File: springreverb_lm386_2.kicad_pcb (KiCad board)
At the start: 2 copper layers, 69.9 x 55.3 mm, 49 parts, among them J1 IN, J10 FromSW, J13 FromGND, J14 From, J15 VR_3_1, J16 VR4_1, J2 Vin, J3 GND, J4 VR1_3, J5 toC6, J6 toC7, J7 VR2_3, J8 VR_2_2, J9 To, U1 TL072, U2 TC1044S, U3 LM386

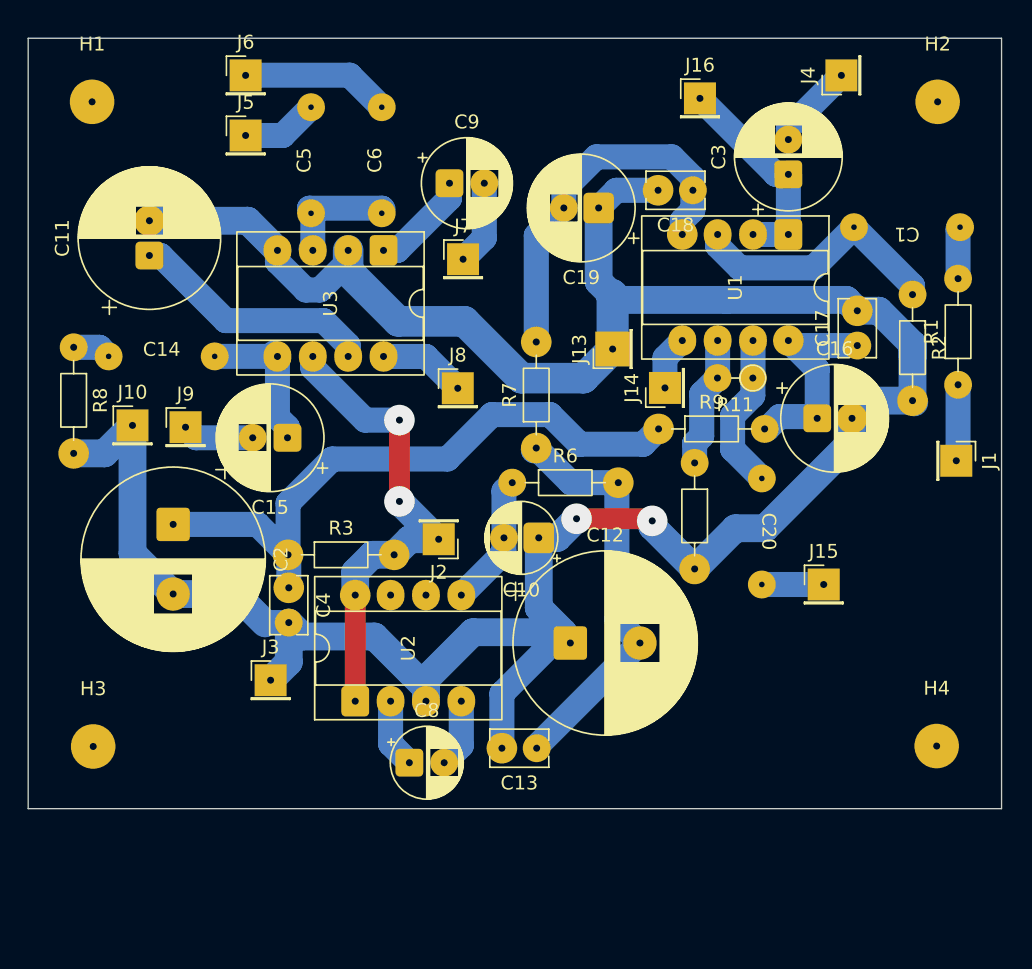
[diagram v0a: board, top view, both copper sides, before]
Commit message: 一旦配置完了
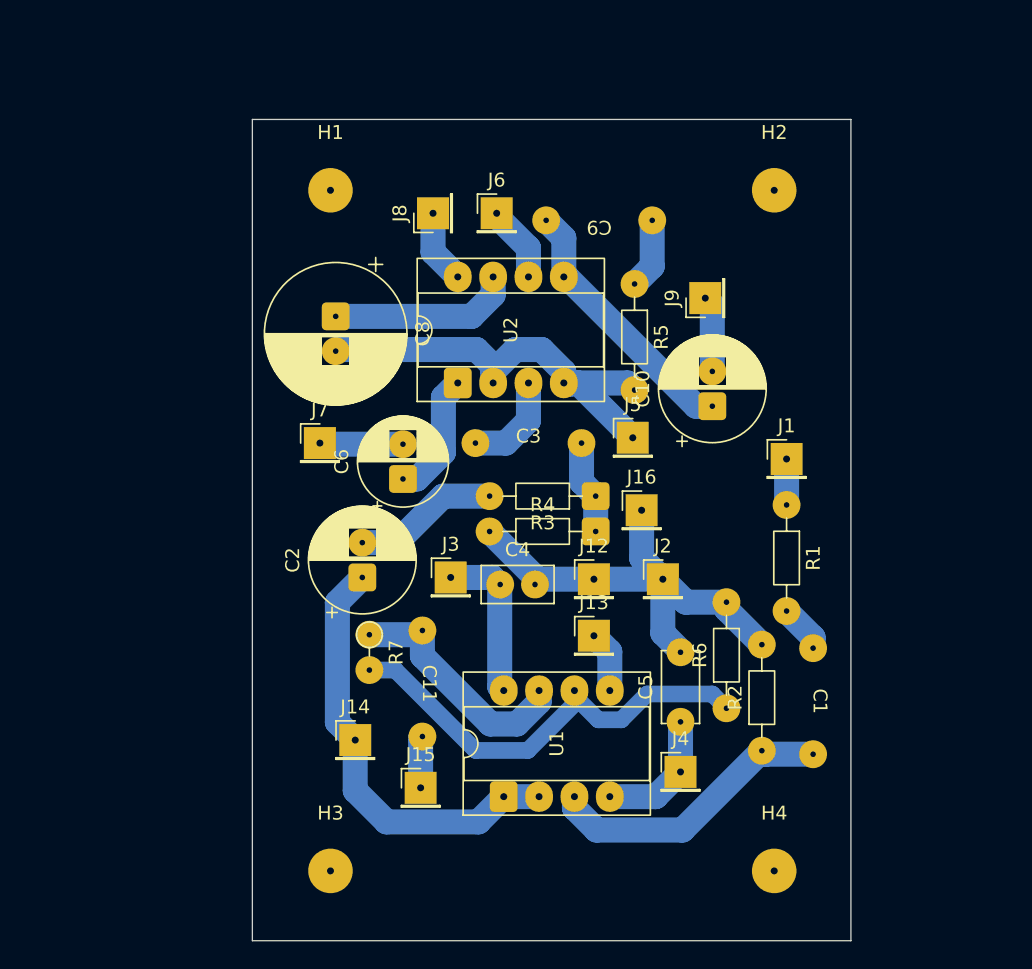
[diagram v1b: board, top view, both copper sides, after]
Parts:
- removed C12: 1000u, Capacitor_THT:CP_Radial_D13.0mm_P5.00mm
- removed C13, C17, C18: 0.1u, Capacitor_THT:C_Rect_L4.0mm_W2.5mm_P2.50mm
- removed C14: 0.047u, MyLibrary:9.3_4.3_p7.5
- removed C15, C16, C19: 100u, Capacitor_THT:CP_Radial_D7.5mm_P2.50mm
- removed C20: 0.022uF, MyLibrary:9.3_4.3_p7.5
- removed J10: FromSW, MyLibrary:PinHeader_1x01_P2.54mm_Vertical
- removed R10: 2.2k, Resistor_THT:R_Axial_DIN0204_L3.6mm_D1.6mm_P7.62mm_Horizontal
- removed R11: 220k, Resistor_THT:R_Axial_DIN0204_L3.6mm_D1.6mm_P2.54mm_Vertical
- removed R8: 10, Resistor_THT:R_Axial_DIN0204_L3.6mm_D1.6mm_P7.62mm_Horizontal
- removed R9: 470, Resistor_THT:R_Axial_DIN0204_L3.6mm_D1.6mm_P7.62mm_Horizontal
- removed U3: LM386, MyLibrary:CERDIP-8_W7.62mm_SideBrazed_Socket
- added J12: FromGND, MyLibrary:PinHeader_1x01_P2.54mm_Vertical, F.Cu at (89.5, 105.0)
- added R4: 4k, Resistor_THT:R_Axial_DIN0204_L3.6mm_D1.6mm_P7.62mm_Horizontal, F.Cu at (82.0, 101.6)
- added R5: 10, Resistor_THT:R_Axial_DIN0204_L3.6mm_D1.6mm_P7.62mm_Horizontal, F.Cu at (92.5, 83.8)
- C10: value 10u -> 100u; footprint Capacitor_THT:CP_Radial_D5.0mm_P2.50mm -> Capacitor_THT:CP_Radial_D7.5mm_P2.50mm
- C11: value 100u -> 0.022uF; footprint Capacitor_THT:CP_Radial_D10.0mm_P2.50mm -> MyLibrary:9.3_4.3_p7.5
- C2: value 1000u -> 100u; footprint Capacitor_THT:CP_Radial_D13.0mm_P5.00mm -> Capacitor_THT:CP_Radial_D7.5mm_P2.50mm
- C3: value 100u -> 470p; footprint Capacitor_THT:CP_Radial_D7.5mm_P2.50mm -> MyLibrary:9.3_4.3_p7.5
- C4: footprint Capacitor_THT:C_Rect_L4.0mm_W2.5mm_P2.50mm -> Capacitor_THT:C_Disc_D5.0mm_W2.5mm_P2.50mm
- C5: value 4700p -> 0.1u; footprint MyLibrary:9.3_4.3_p7.5 -> Capacitor_THT:C_Disc_D5.0mm_W2.5mm_P5.00mm
- C6: value 470p -> 10u; footprint MyLibrary:9.3_4.3_p7.5 -> Capacitor_THT:CP_Radial_D6.3mm_P2.50mm
- C8: value 10u -> 100u; footprint Capacitor_THT:CP_Radial_D5.0mm_P2.50mm -> Capacitor_THT:CP_Radial_D10.0mm_P2.50mm
- C9: value 10u -> 0.047u; footprint Capacitor_THT:CP_Radial_D6.3mm_P2.50mm -> MyLibrary:9.3_4.3_p7.5
- J13: value FromGND -> From
- J14: value From -> VR4_1
- J15: value VR_3_1 -> VR4_3
- J16: value VR4_1 -> OUT_GND
- J2: value Vin -> IN_GND
- J3: value GND -> +15v
- J4: value VR1_3 -> -15v
- J5: value toC6 -> GND2
- J6: value toC7 -> +15v2
- R3: value 10 -> 10k
- R6: value 10 -> 2.2k
- R7: value 470 -> 220k; footprint Resistor_THT:R_Axial_DIN0204_L3.6mm_D1.6mm_P7.62mm_Horizontal -> Resistor_THT:R_Axial_DIN0204_L3.6mm_D1.6mm_P2.54mm_Vertical
- U2: value TC1044S -> LM386
- moved J4 51.4 mm to (95.8, 118.9), turned to 0 degrees
- moved C5 48.3 mm to (95.8, 115.3)
- moved U1 45.3 mm to (83.1, 120.7), turned to 90 degrees
- moved J9 38.5 mm to (97.5, 84.8), turned to 90 degrees
- moved C11 36.5 mm to (77.2, 112.5), turned to -90 degrees
- moved J5 35.3 mm to (92.3, 94.9)
- moved C1 34.7 mm to (105.3, 113.8), turned to -90 degrees
- moved R2 34.5 mm to (101.6, 117.3), turned to 90 degrees
- moved J14 33.7 mm to (72.4, 116.6), turned to 0 degrees
- moved C8 32.5 mm to (71.0, 86.1), turned to -90 degrees
- moved J15 32.4 mm to (77.1, 120.0)
- moved J16 29.9 mm to (93.0, 100.1)
- moved C3 26.9 mm to (84.8, 95.2), turned to 0 degrees
- moved U2 24.0 mm to (79.8, 90.9)
- moved C6 23.0 mm to (75.8, 97.8)
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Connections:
- C10 pad 1: GND -> Net-(C10-Pad1)
- C10 pad 2: Net-(U2-VOUT) -> Net-(J10-In)
- C11 pad 1: Net-(U3-BYPASS) -> Net-(C11-Pad1)
- C11 pad 2: GND -> Net-(J15-Pin_1)
- C2 pad 1: Net-(C2-Pad1) -> Net-(J14-Pin_1)
- C2 pad 2: GND -> Net-(C2-Pad2)
- C3 pad 1: Net-(J16-Pin_1) -> Net-(U2-+)
- C3 pad 2: Net-(J4-Pin_1) -> Net-(C3-Pad2)
- C4 pad 1: Net-(C2-Pad1) -> Net-(J3-Pin_1)
- C4 pad 2: GND -> GND1
- C5 pad 1: Net-(U3-+) -> Net-(J4-Pin_1)
- C5 pad 2: Net-(J5-Pin_1) -> GND1
- C6 pad 1: Net-(U3-+) -> Net-(C6-Pad1)
- C6 pad 2: Net-(J6-Pin_1) -> Net-(J7-Pin_1)
- C8 pad 1: Net-(U2-CAP+) -> Net-(U2-BYPASS)
- C8 pad 2: Net-(U2-CAP-) -> GND2
- C9 pad 2: Net-(J7-Pin_1) -> Net-(C10-Pad1)
- J13 pad 1: GND -> Net-(J11-In)
- J14 pad 1: Net-(J12-In) -> Net-(J14-Pin_1)
- J16 pad 1: Net-(J16-Pin_1) -> GND1
- J2 pad 1: Net-(J2-Pin_1) -> GND1
- J3 pad 1: GND -> Net-(J3-Pin_1)
- J5 pad 1: Net-(J5-Pin_1) -> GND2
- J9 pad 1: Net-(J11-In) -> Net-(J10-In)
- R2 pad 2: GND -> GND1
- R3 pad 1: Net-(C2-Pad1) -> Net-(C3-Pad2)
- R3 pad 2: Net-(J2-Pin_1) -> Net-(C2-Pad2)
- R6 pad 1: Net-(U2-VOUT) -> Net-(U1B--)
- R6 pad 2: Net-(C12-Pad2) -> GND1
- R7 pad 1: Net-(C12-Pad2) -> Net-(C11-Pad1)
- R7 pad 2: Net-(U1C-V-) -> Net-(U1B--)
- U1 pad 1: Net-(J16-Pin_1) -> Net-(J14-Pin_1)
- U1 pad 2: Net-(J16-Pin_1) -> Net-(J14-Pin_1)
- U1 pad 4: Net-(U1C-V-) -> Net-(J4-Pin_1)
- U1 pad 5: Net-(J12-In) -> Net-(J11-In)
- U1 pad 7: Net-(C20-Pad1) -> Net-(C11-Pad1)
- U1 pad 8: Net-(U1C-V+) -> Net-(J3-Pin_1)
- U2 pad 1: Net-(J2-Pin_1) -> Net-(C6-Pad1)
- U2 pad 2: Net-(U2-CAP+) -> GND2
- U2 pad 3: GND -> Net-(U2-+)
- U2 pad 4: Net-(U2-CAP-) -> GND2
- U2 pad 5: Net-(U2-VOUT) -> Net-(C10-Pad1)
- U2 pad 6: unconnected-(U2-LV-Pad6) -> Net-(J6-Pin_1)
- U2 pad 7: unconnected-(U2-OSC-Pad7) -> Net-(U2-BYPASS)
- U2 pad 8: Net-(J2-Pin_1) -> Net-(J8-Pin_1)
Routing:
- net GND: track 197.5 -> 0.00 mm, vias 2 -> 0
- net Net-(C2-Pad1): track 45.8 -> 0.00 mm
- net GND1: track 0.00 -> 35.4 mm
- net Net-(J2-Pin_1): track 34.6 -> 0.00 mm, vias 2 -> 0
- net GND2: track 0.00 -> 33.7 mm
- net Net-(J14-Pin_1): track 0.00 -> 31.5 mm
- net Net-(C12-Pad2): track 30.4 -> 0.00 mm
- net Net-(U1C-V-): track 27.0 -> 0.00 mm
- net Net-(U1B--): track 9.47 -> 32.7 mm
- net Net-(C10-Pad1): track 0.00 -> 19.1 mm
- net Net-(U3-BYPASS): track 17.8 -> 0.00 mm
- net Net-(C11-Pad1): track 0.00 -> 17.6 mm
- net Net-(J16-Pin_1): track 15.5 -> 0.00 mm
- net Net-(U1C-V+): track 15.2 -> 0.00 mm
- net Net-(U2-BYPASS): track 0.00 -> 13.2 mm
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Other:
- board size 69.9 x 55.3 mm -> 43 x 59 mm

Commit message: 配置を修正
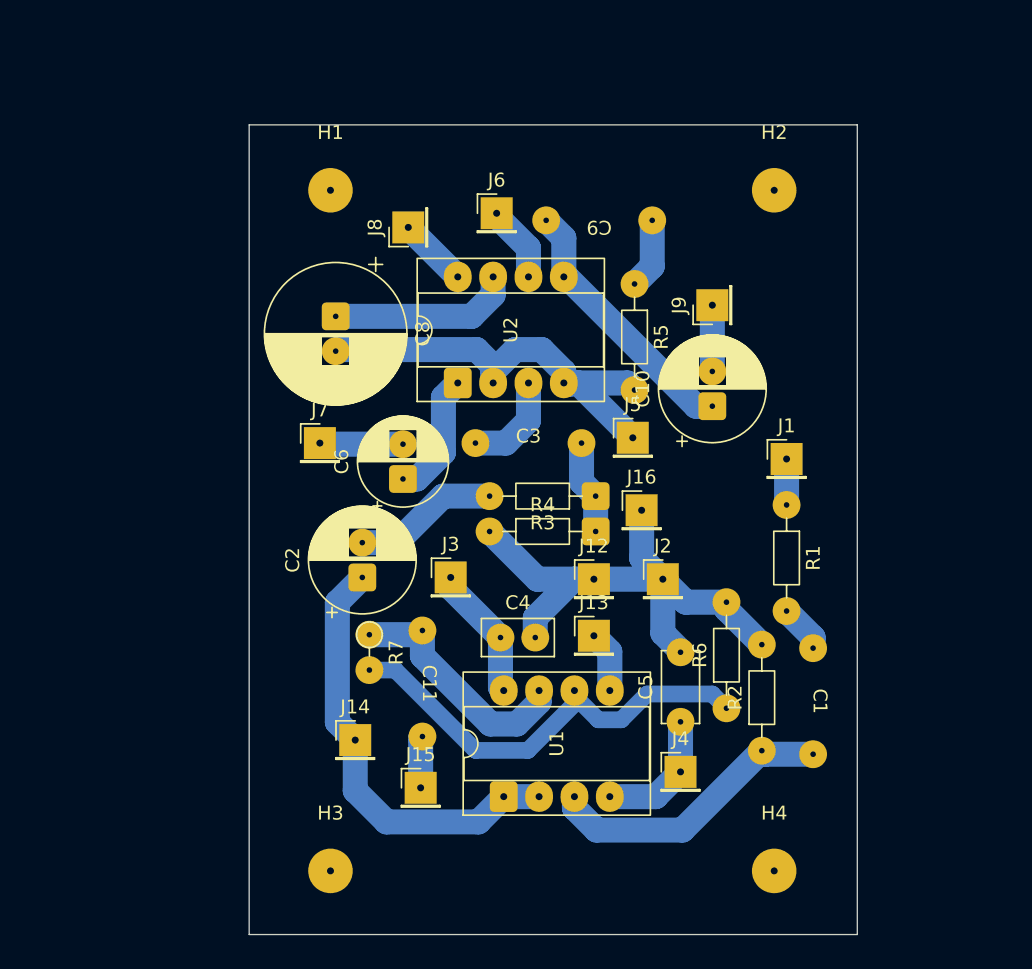
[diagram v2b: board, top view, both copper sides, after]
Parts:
- moved C4 3.81 mm to (82.8, 109.2)
- moved J8 2.05 mm to (76.2, 79.8)
- moved J9 0.72 mm to (98.0, 85.3)
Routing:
- net GND1: track 35.4 -> 41.5 mm
- net Net-(J3-Pin_1): track 11.5 -> 9.71 mm
- net Net-(J10-In): track 5.48 -> 4.76 mm
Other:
- board size 43 x 59 mm -> 43.7 x 58.2 mm
